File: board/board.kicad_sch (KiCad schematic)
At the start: 10 parts, among them J1 Raspberry_Pi_4

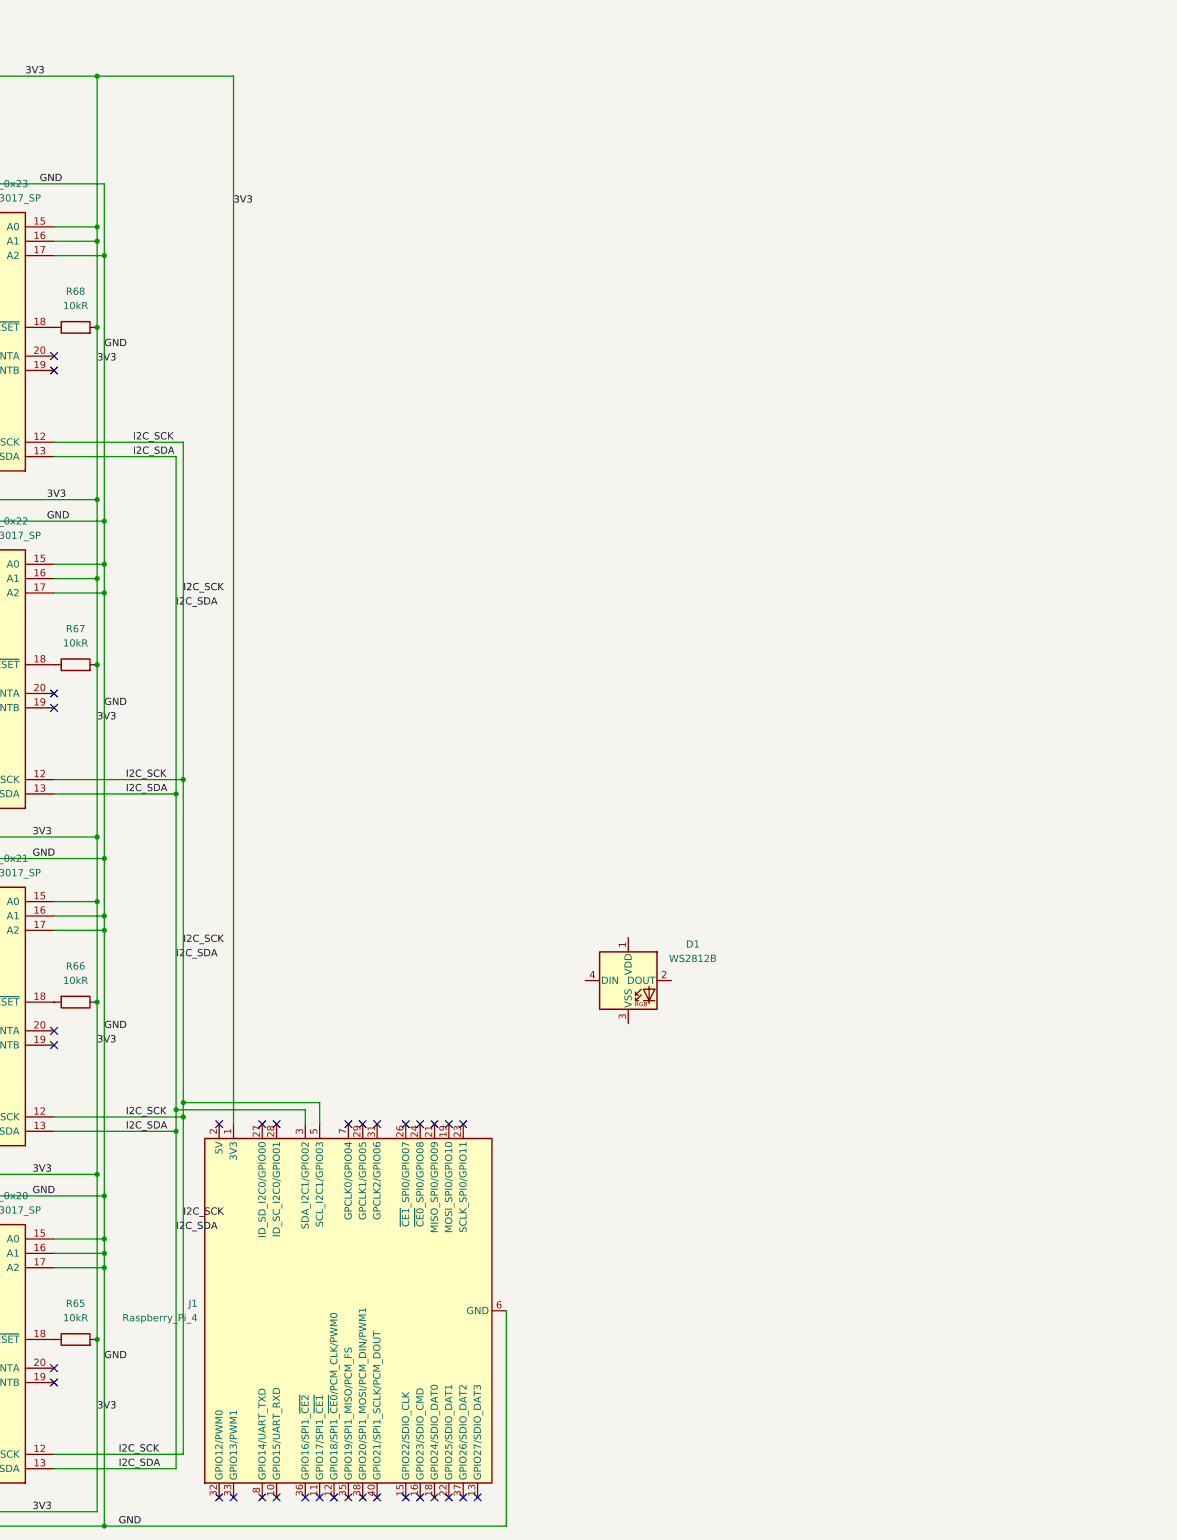
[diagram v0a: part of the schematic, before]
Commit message: just a few adjustments left
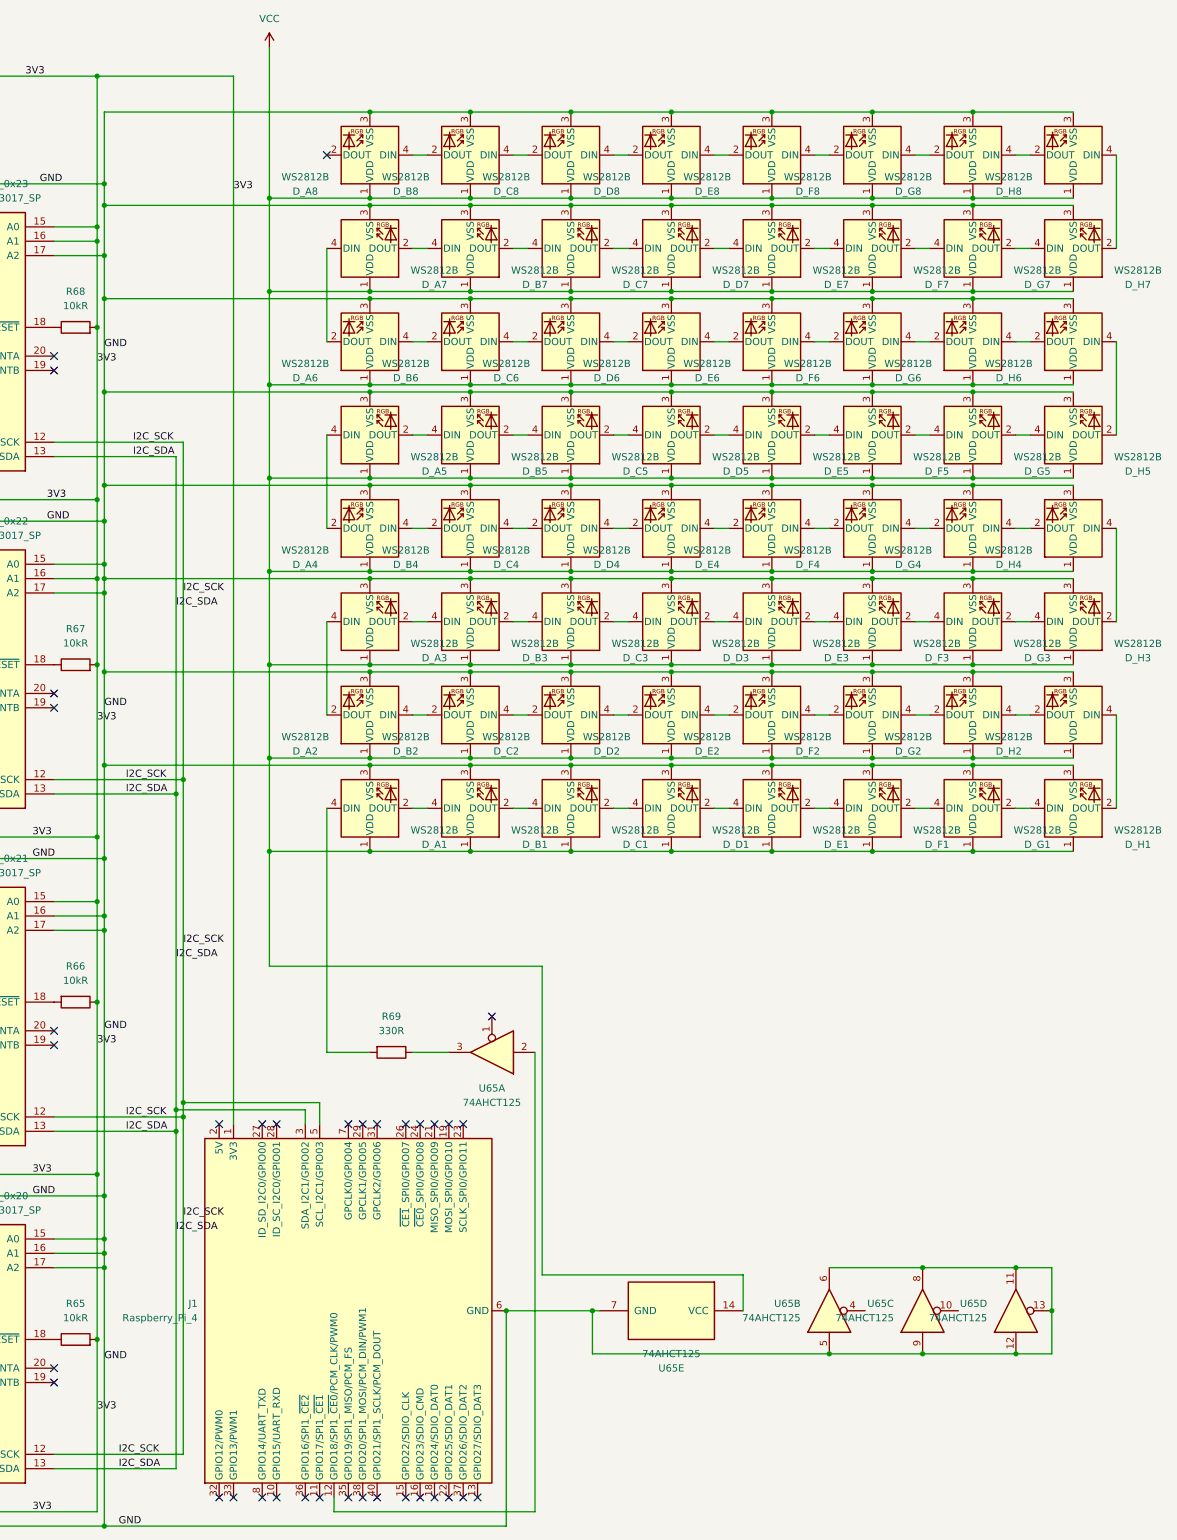
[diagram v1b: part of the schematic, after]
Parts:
- added D_A2, D_A3, D_A4, D_A5, D_A6, D_A7, D_A8, D_B1, D_B2, D_B3, D_B4, D_B5, D_B6, D_B7, D_B8, D_C1, D_C2, D_C3, D_C4, D_C5, D_C6, D_C7, D_C8, D_D1, D_D2, D_D3, D_D4, D_D5, D_D6, D_D7, D_D8, D_E1, D_E2, D_E3, D_E4, D_E5, D_E6, D_E7, D_E8, D_F1, D_F2, D_F3, D_F4, D_F5, D_F6, D_F7, D_F8, D_G1, D_G2, D_G3, D_G4, D_G5, D_G6, D_G7, D_G8, D_H1, D_H2, D_H3, D_H4, D_H5, D_H6, D_H7, D_H8: WS2812B, LED_SMD:LED_WS2812B_PLCC4_5.0x5.0mm_P3.2mm, symbol LED:WS2812B
- added R69: 330R, symbol Device:R
- added U65: 74AHCT125, symbol 74xx:74AHCT125
- renumbered D1 to D_A1
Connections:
- net GND: now also D_A1.3 (VSS), D_A2.3 (VSS), D_A3.3 (VSS), D_A4.3 (VSS), D_A5.3 (VSS), D_A6.3 (VSS), D_A7.3 (VSS), D_A8.3 (VSS), D_B1.3 (VSS), D_B2.3 (VSS), D_B3.3 (VSS), D_B4.3 (VSS), D_B5.3 (VSS), D_B6.3 (VSS), D_B7.3 (VSS), D_B8.3 (VSS), D_C1.3 (VSS), D_C2.3 (VSS), D_C3.3 (VSS), D_C4.3 (VSS), D_C5.3 (VSS), D_C6.3 (VSS), D_C7.3 (VSS), D_C8.3 (VSS), D_D1.3 (VSS), D_D2.3 (VSS), D_D3.3 (VSS), D_D4.3 (VSS), D_D5.3 (VSS), D_D6.3 (VSS), D_D7.3 (VSS), D_D8.3 (VSS), D_E1.3 (VSS), D_E2.3 (VSS), D_E3.3 (VSS), D_E4.3 (VSS), D_E5.3 (VSS), D_E6.3 (VSS), D_E7.3 (VSS), D_E8.3 (VSS), D_F1.3 (VSS), D_F2.3 (VSS), D_F3.3 (VSS), D_F4.3 (VSS), D_F5.3 (VSS), D_F6.3 (VSS), D_F7.3 (VSS), D_F8.3 (VSS), D_G1.3 (VSS), D_G2.3 (VSS), D_G3.3 (VSS), D_G4.3 (VSS), D_G5.3 (VSS), D_G6.3 (VSS), D_G7.3 (VSS), D_G8.3 (VSS), D_H1.3 (VSS), D_H2.3 (VSS), D_H3.3 (VSS), D_H4.3 (VSS), D_H5.3 (VSS), D_H6.3 (VSS), D_H7.3 (VSS), D_H8.3 (VSS), U65.11, U65.12, U65.13, U65.5, U65.6, U65.7 (GND), U65.8, U65.9
- net VCC: now reaches D_A1.1 (VDD)
- net VCC: now also D_A2.1 (VDD), D_A3.1 (VDD), D_A4.1 (VDD), D_A5.1 (VDD), D_A6.1 (VDD), D_A7.1 (VDD), D_A8.1 (VDD), D_B1.1 (VDD), D_B2.1 (VDD), D_B3.1 (VDD), D_B4.1 (VDD), D_B5.1 (VDD), D_B6.1 (VDD), D_B7.1 (VDD), D_B8.1 (VDD), D_C1.1 (VDD), D_C2.1 (VDD), D_C3.1 (VDD), D_C4.1 (VDD), D_C5.1 (VDD), D_C6.1 (VDD), D_C7.1 (VDD), D_C8.1 (VDD), D_D1.1 (VDD), D_D2.1 (VDD), D_D3.1 (VDD), D_D4.1 (VDD), D_D5.1 (VDD), D_D6.1 (VDD), D_D7.1 (VDD), D_D8.1 (VDD), D_E1.1 (VDD), D_E2.1 (VDD), D_E3.1 (VDD), D_E4.1 (VDD), D_E5.1 (VDD), D_E6.1 (VDD), D_E7.1 (VDD), D_E8.1 (VDD), D_F1.1 (VDD), D_F2.1 (VDD), D_F3.1 (VDD), D_F4.1 (VDD), D_F5.1 (VDD), D_F6.1 (VDD), D_F7.1 (VDD), D_F8.1 (VDD), D_G1.1 (VDD), D_G2.1 (VDD), D_G3.1 (VDD), D_G4.1 (VDD), D_G5.1 (VDD), D_G6.1 (VDD), D_G7.1 (VDD), D_G8.1 (VDD), D_H1.1 (VDD), D_H2.1 (VDD), D_H3.1 (VDD), D_H4.1 (VDD), D_H5.1 (VDD), D_H6.1 (VDD), D_H7.1 (VDD), D_H8.1 (VDD), U65.14 (VCC)
- net at D_A1.2 (DOUT): now also D_B1.4 (DIN)
- net at D_A1.4 (DIN): now also R69.2
- net at J1.12 (GPIO18/SPI1_~{CE0}/PCM_CLK/PWM0): now also U65.2
- new net: D_G6.4 (DIN), D_H6.2 (DOUT)
- new net: D_H5.2 (DOUT), D_H6.4 (DIN)
- new net: D_G1.2 (DOUT), D_H1.4 (DIN)
- new net: D_F1.2 (DOUT), D_G1.4 (DIN)
- new net: D_D6.4 (DIN), D_E6.2 (DOUT)
- new net: D_E6.4 (DIN), D_F6.2 (DOUT)
- new net: D_B2.4 (DIN), D_C2.2 (DOUT)
- new net: D_C2.4 (DIN), D_D2.2 (DOUT)
- new net: D_F7.2 (DOUT), D_G7.4 (DIN)
- new net: D_E7.2 (DOUT), D_F7.4 (DIN)
- new net: D_A4.4 (DIN), D_B4.2 (DOUT)
- new net: D_B4.4 (DIN), D_C4.2 (DOUT)
- new net: D_D4.4 (DIN), D_E4.2 (DOUT)
- new net: D_E4.4 (DIN), D_F4.2 (DOUT)
- new net: D_D2.4 (DIN), D_E2.2 (DOUT)
- new net: D_B6.4 (DIN), D_C6.2 (DOUT)
- new net: D_C6.4 (DIN), D_D6.2 (DOUT)
- new net: D_E1.2 (DOUT), D_F1.4 (DIN)
- new net: D_D1.2 (DOUT), D_E1.4 (DIN)
- new net: D_D7.2 (DOUT), D_E7.4 (DIN)
- new net: D_E8.4 (DIN), D_F8.2 (DOUT)
- new net: D_F8.4 (DIN), D_G8.2 (DOUT)
- new net: D_F4.4 (DIN), D_G4.2 (DOUT)
- new net: D_C7.2 (DOUT), D_D7.4 (DIN)
- new net: D_B7.2 (DOUT), D_C7.4 (DIN)
- new net: D_A5.2 (DOUT), D_B5.4 (DIN)
- new net: D_A4.2 (DOUT), D_A5.4 (DIN)
- new net: D_G5.2 (DOUT), D_H5.4 (DIN)
- new net: D_G8.4 (DIN), D_H8.2 (DOUT)
- new net: D_H7.2 (DOUT), D_H8.4 (DIN)
- new net: D_A2.4 (DIN), D_B2.2 (DOUT)
- new net: D_G3.2 (DOUT), D_H3.4 (DIN)
- new net: D_F3.2 (DOUT), D_G3.4 (DIN)
- new net: D_A7.2 (DOUT), D_B7.4 (DIN)
- new net: D_F6.4 (DIN), D_G6.2 (DOUT)
- new net: D_H3.2 (DOUT), D_H4.4 (DIN)
- new net: D_A8.4 (DIN), D_B8.2 (DOUT)
- new net: D_G4.4 (DIN), D_H4.2 (DOUT)
- new net: D_E3.2 (DOUT), D_F3.4 (DIN)
- new net: D_C5.2 (DOUT), D_D5.4 (DIN)
- new net: D_B5.2 (DOUT), D_C5.4 (DIN)
- new net: D_A2.2 (DOUT), D_A3.4 (DIN)
- new net: D_C8.4 (DIN), D_D8.2 (DOUT)
- new net: D_D8.4 (DIN), D_E8.2 (DOUT)
- new net: D_F2.4 (DIN), D_G2.2 (DOUT)
- new net: D_G2.4 (DIN), D_H2.2 (DOUT)
- new net: D_B8.4 (DIN), D_C8.2 (DOUT)
- new net: R69.1, U65.3
- new net: D_B3.2 (DOUT), D_C3.4 (DIN)
- new net: D_A3.2 (DOUT), D_B3.4 (DIN)
- new net: D_A6.2 (DOUT), D_A7.4 (DIN)
- new net: D_E5.2 (DOUT), D_F5.4 (DIN)
- new net: D_D5.2 (DOUT), D_E5.4 (DIN)
- new net: D_G7.2 (DOUT), D_H7.4 (DIN)
- new net: D_A6.4 (DIN), D_B6.2 (DOUT)
- new net: D_F5.2 (DOUT), D_G5.4 (DIN)
- new net: D_H1.2 (DOUT), D_H2.4 (DIN)
- new net: D_C3.2 (DOUT), D_D3.4 (DIN)
- new net: D_D3.2 (DOUT), D_E3.4 (DIN)
- new net: D_E2.4 (DIN), D_F2.2 (DOUT)
- new net: D_C1.2 (DOUT), D_D1.4 (DIN)
- new net: D_B1.2 (DOUT), D_C1.4 (DIN)
- new net: D_C4.4 (DIN), D_D4.2 (DOUT)
- no-connect marks 35 -> 36
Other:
- moved on the sheet: D_A1
